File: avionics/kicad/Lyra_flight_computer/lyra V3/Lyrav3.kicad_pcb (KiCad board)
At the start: 4 copper layers, 25 x 55 mm, 84 parts, among them J2 Screw_Terminal_01x06, J3 Conn_01x02, J4 Conn_01x02, J6 Conn_01x06, J7 USB_B_Micro, J8 Conn_01x04, J9 Screw_Terminal_01x06, Q1 AO3401A, Q2 AO3400A, Q3 AO3400A, Q4 AO3400A, Q5 AO3400A, U1 AZ1117-3.3, U2 BMI088, U3 MPL3115A2, U4 ADXL375BCCZ-RL7, U5 LIS3MDL, U6 ADS1015IDGS, U7 W25Q64JVXGIQ, U8 RP2040, X1 S3D12.288000B20F30T

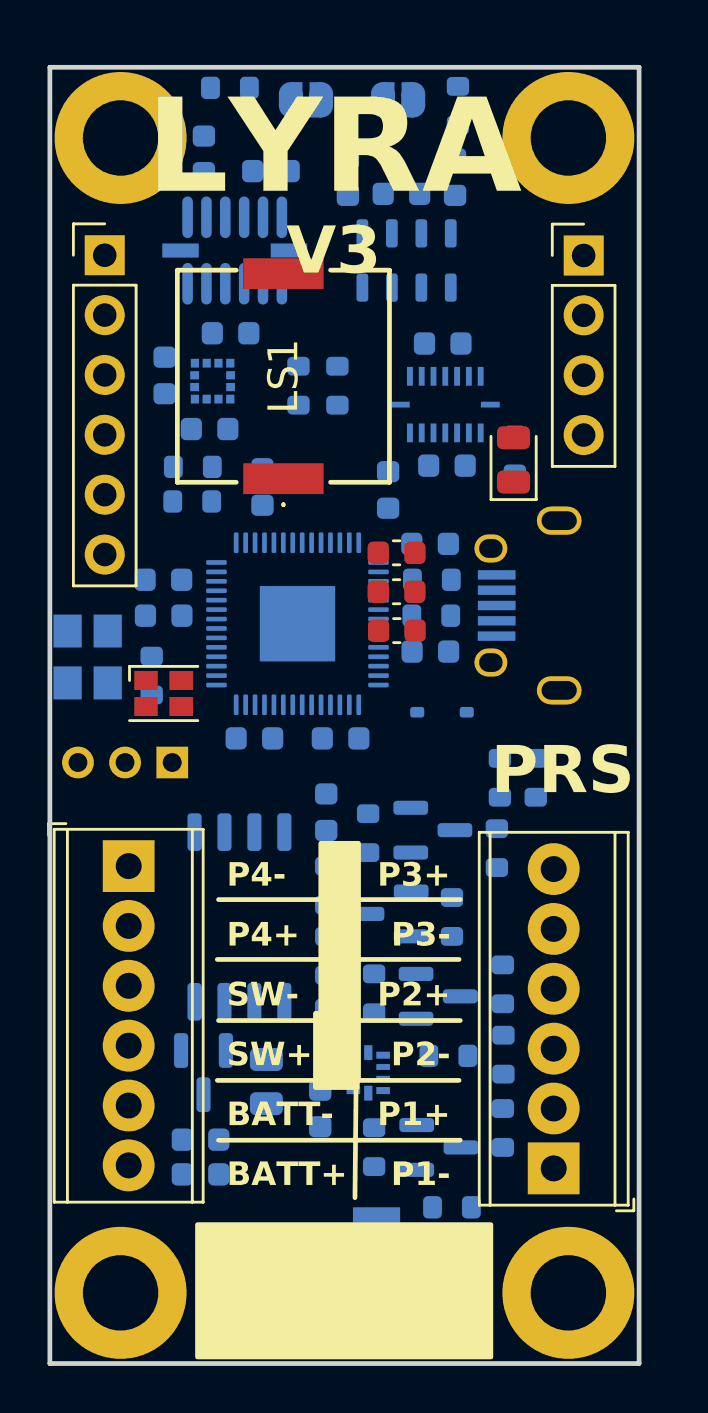
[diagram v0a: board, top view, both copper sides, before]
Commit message: routing twioce
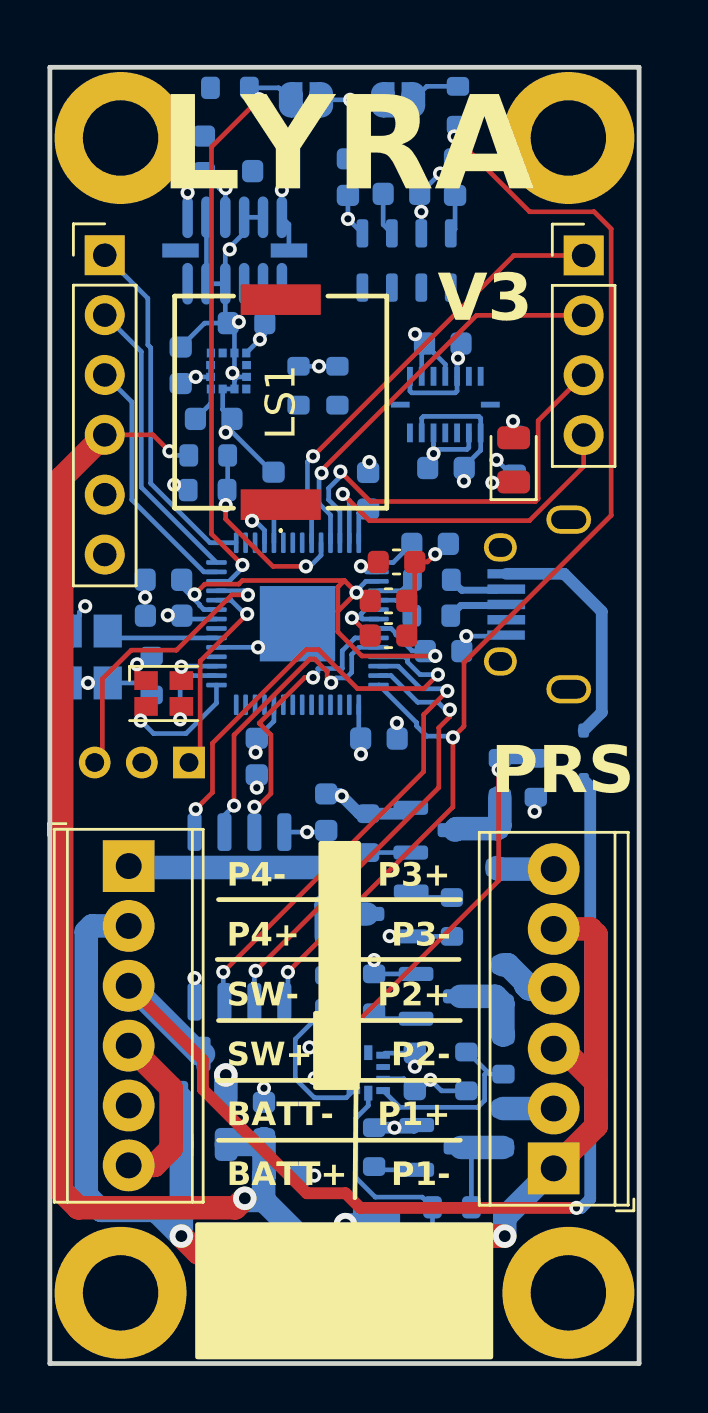
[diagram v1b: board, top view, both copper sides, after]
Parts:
- moved D3 6.28 mm to (206.2, 93.2), turned to 90 degrees
- moved C15 4.31 mm to (199.1, 106.6)
- moved F1 3.75 mm to (190.1, 109.7), turned to 0 degrees
- moved C7 3.45 mm to (193.4, 111.0), turned to 0 degrees
- moved C8 2.81 mm to (192.7, 108.7), turned to 90 degrees
- moved C22 1.63 mm to (197.6, 92.5), turned to 0 degrees
- moved LS1 1.11 mm to (193.4, 78.2)
- moved R24 1.01 mm to (201.3, 106.6), turned to -90 degrees
- moved C21 0.85 mm to (197.1, 82.0)
- moved R5 0.81 mm to (190.3, 82.0)
- moved R4 0.81 mm to (190.3, 80.5)
- moved C13 0.80 mm to (191.9, 74.9)
- moved U5 0.80 mm to (191.2, 76.9)
- moved C12 0.80 mm to (189.1, 76.7)
- moved C23 0.78 mm to (192.4, 93.3), turned to -90 degrees
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- renumbered Je to J5
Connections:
- J2 pad 2: /PYRO PWR -> +12P
- J9 pad 1: /PYRO PWR -> +12P
- J9 pad 3: /PYRO PWR -> +12P
- J9 pad 5: /PYRO PWR -> +12P
- U6 pad 4: /P1 CONT  -> /P2 CONT 
- U6 pad 5: /P2 CONT  -> /P1 CONT 
- U6 pad 6: /P3 CONT  -> /P4 CONT 
- U6 pad 7: /P4 CONT  -> /P3 CONT 
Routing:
- net GND: track 0.00 -> 80.0 mm, vias 0 -> 33
- net +12VA: track 0.00 -> 60.9 mm, vias 0 -> 2
- net +12P: track 0.00 -> 56.7 mm, vias 0 -> 2
- net +3V3: track 0.00 -> 54.0 mm, vias 0 -> 20
- net /QSPI_SS: track 0.00 -> 51.0 mm, vias 0 -> 3
- net +12V: track 0.00 -> 46.6 mm, vias 0 -> 1
- net /RUN: track 0.00 -> 24.6 mm, vias 0 -> 2
- net +1V1: track 0.00 -> 21.8 mm, vias 0 -> 3
- net /QSPI_SD2: track 0.00 -> 20.5 mm, vias 0 -> 2
- net /P3 CONT : track 0.00 -> 19.8 mm, vias 0 -> 2
- net /QSPI_SD1: track 0.00 -> 19.5 mm, vias 0 -> 2
- net /BRKOUT1: track 0.00 -> 18.9 mm, vias 0 -> 1
- net /BRKOUT3: track 0.00 -> 18.4 mm, vias 0 -> 1
- net /QSPI_SDO: track 0.00 -> 18.1 mm, vias 0 -> 2
- net /BRKOUT2: track 0.00 -> 17.2 mm, vias 0 -> 1
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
